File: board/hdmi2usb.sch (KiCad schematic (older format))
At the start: 0 parts

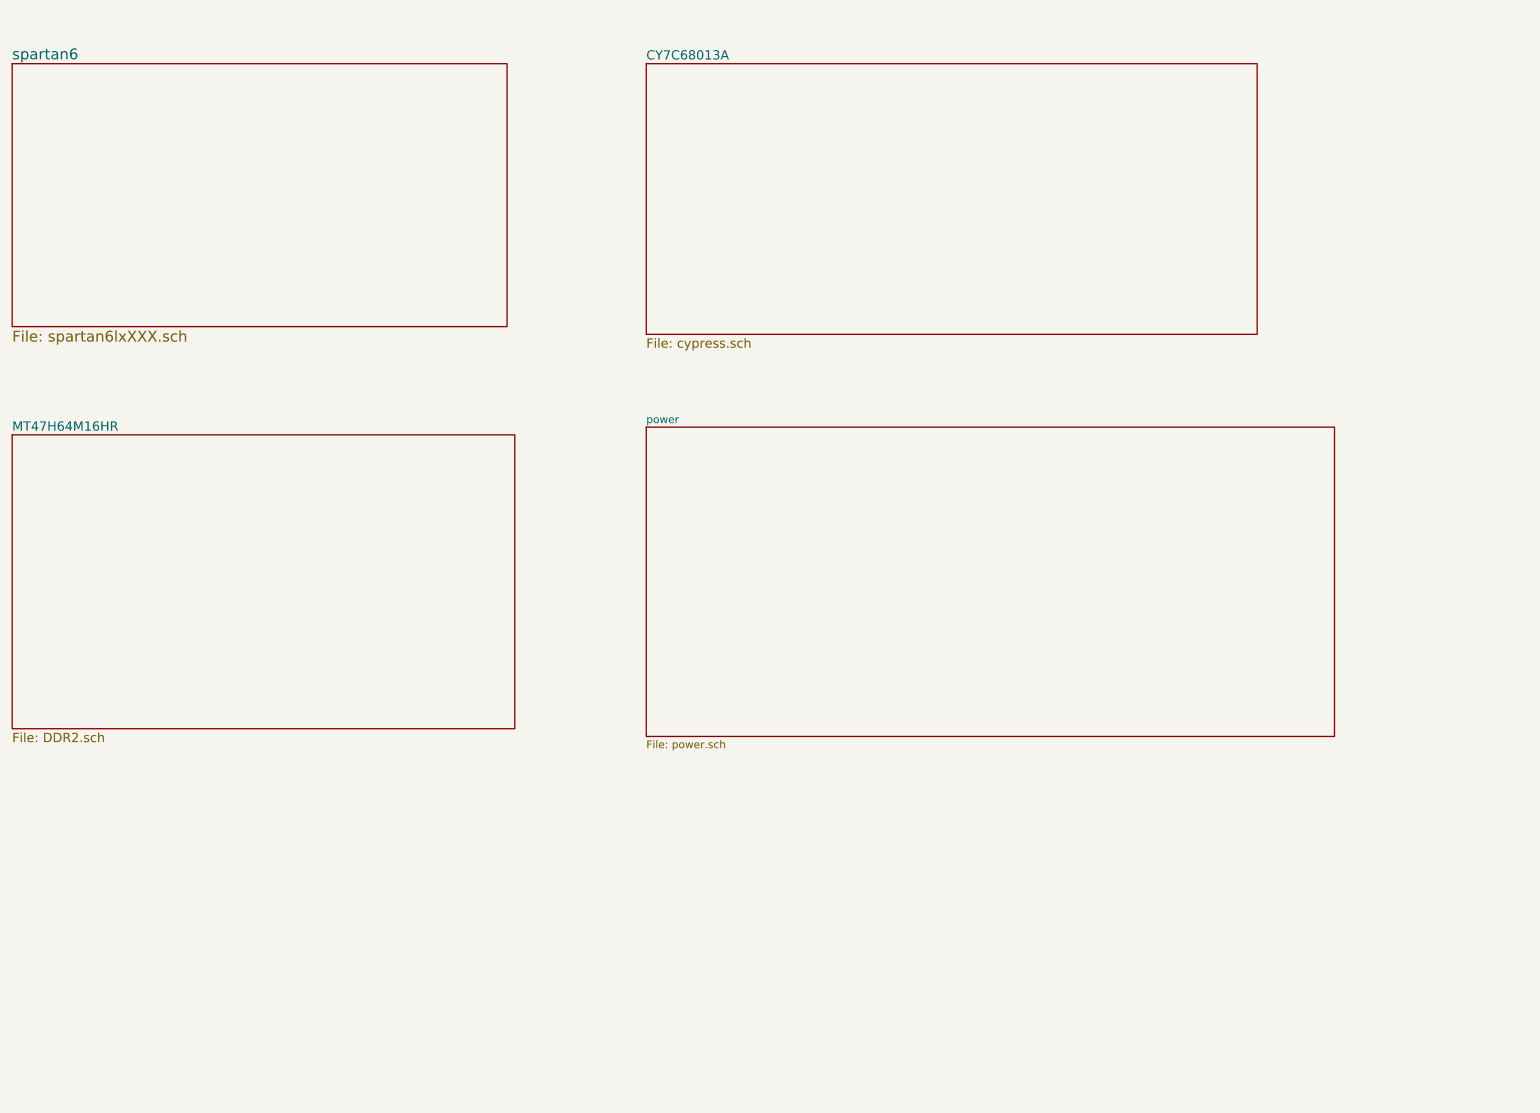
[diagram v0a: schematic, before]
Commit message: Issue #336
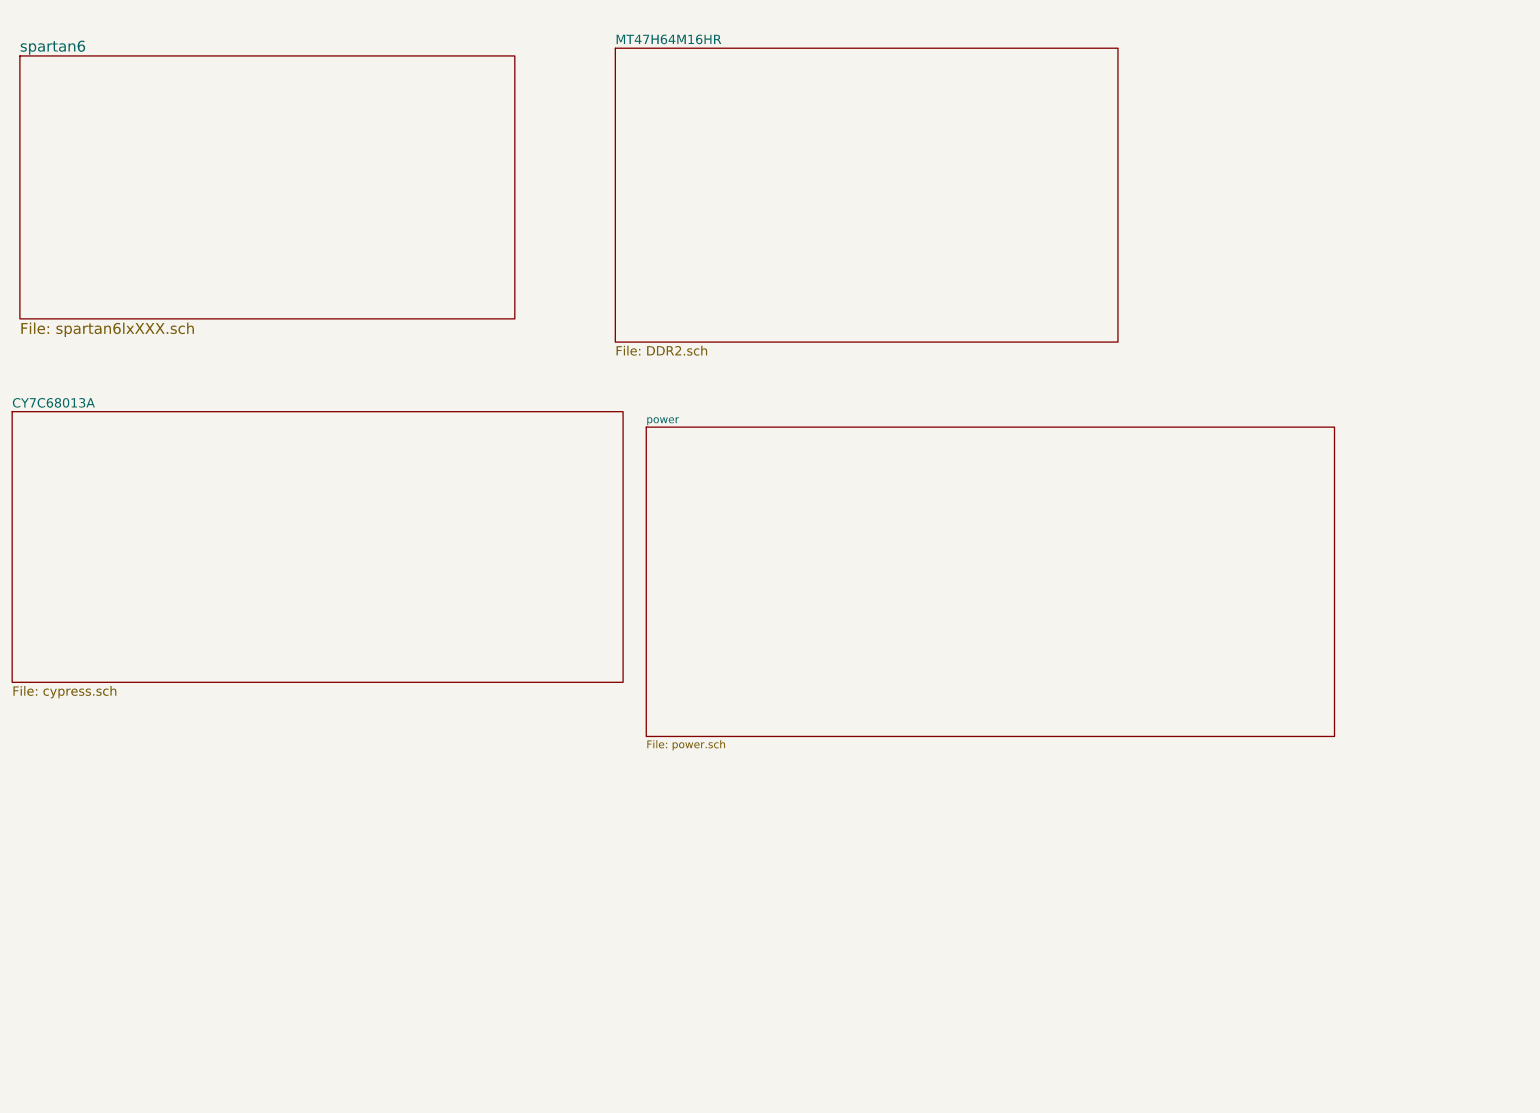
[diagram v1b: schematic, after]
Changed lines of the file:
@@
 Sheet 1 5
 Title ""
-Date "15 jun 2013"
+Date "19 jun 2013"
 Rev ""
 Comp ""
@@
 $EndDescr
 $Sheet
-S 1000 3300 3250 1900
+S 4900 800  3250 1900
 U 51B846F4
 F0 "MT47H64M16HR" 60
@@
 $EndSheet
 $Sheet
-S 5100 900  3950 1750
+S 1000 3150 3950 1750
 U 51B5BBC1
 F0 "CY7C68013A" 60
@@
 $EndSheet
 $Sheet
-S 1000 900  3200 1700
+S 1050 850  3200 1700
 U 51AED6DE
 F0 "spartan6" 70

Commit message: Issue #336
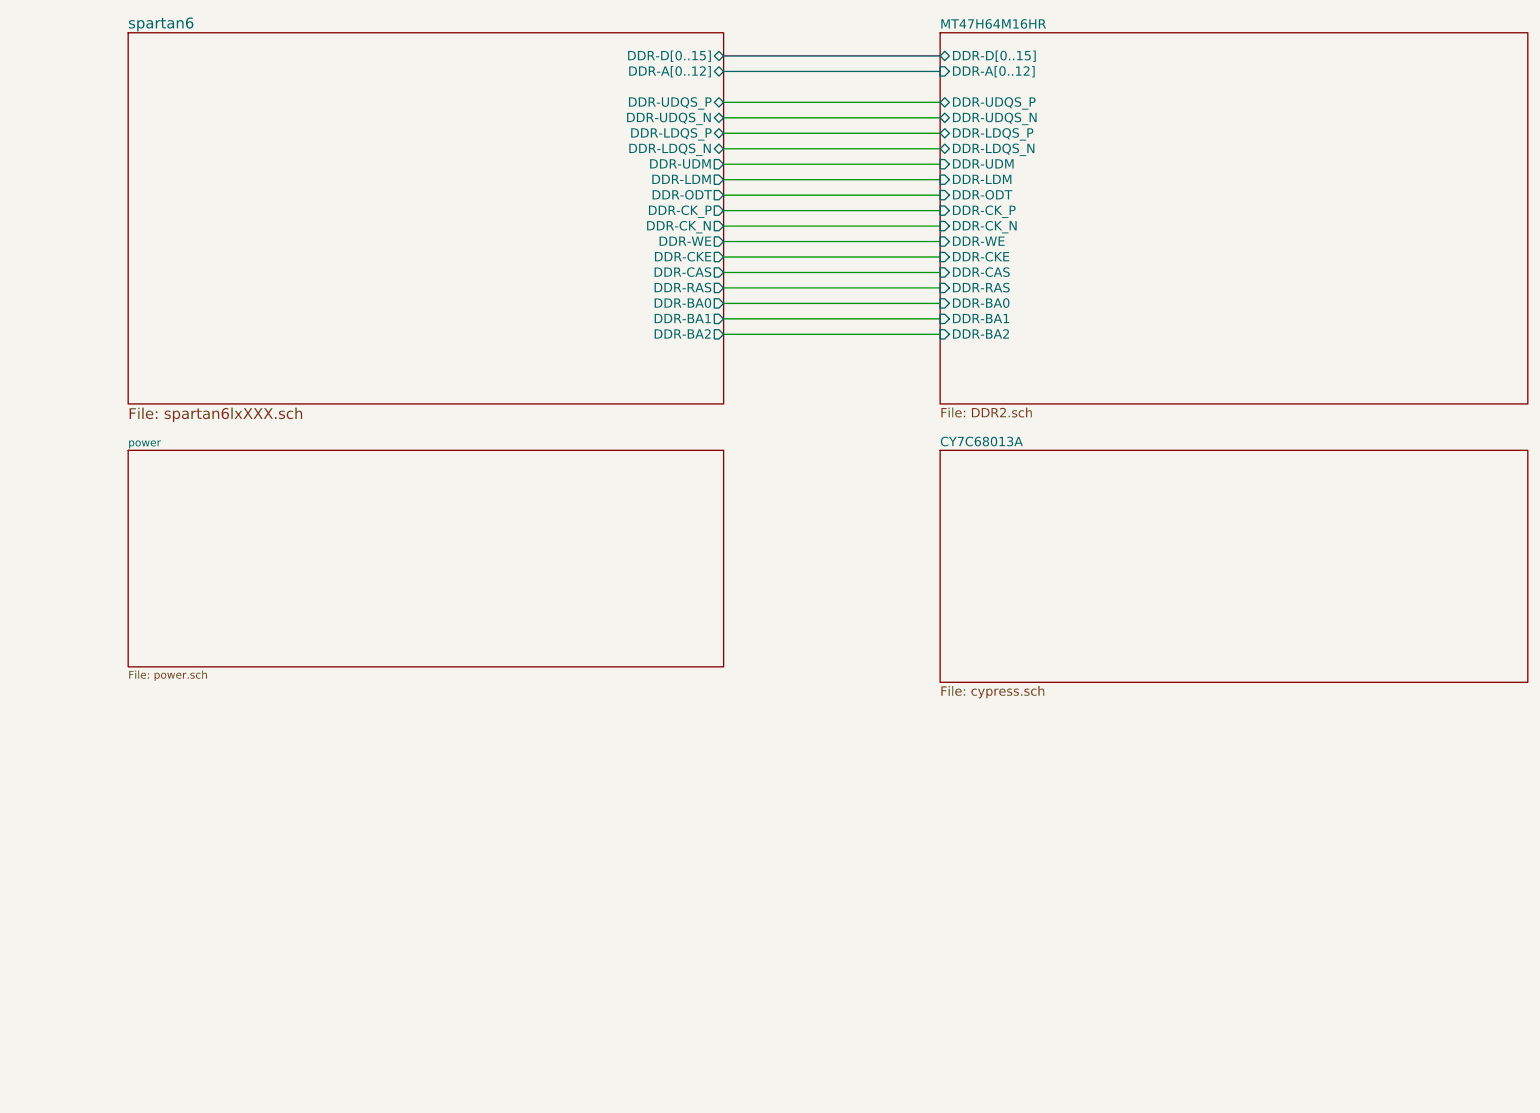
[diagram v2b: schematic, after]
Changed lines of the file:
@@
 Sheet 1 5
 Title ""
-Date "19 jun 2013"
+Date "24 jun 2013"
 Rev ""
 Comp ""
@@
 $EndDescr
 $Sheet
-S 4900 800  3250 1900
-U 51B846F4
-F0 "MT47H64M16HR" 60
-F1 "DDR2.sch" 60
-$EndSheet
-$Sheet
-S 1000 3150 3950 1750
+S 7000 3400 3800 1500
 U 51B5BBC1
 F0 "CY7C68013A" 60
@@
 $EndSheet
 $Sheet
-S 1050 850  3200 1700
-U 51AED6DE
-F0 "spartan6" 70
-F1 "spartan6lxXXX.sch" 70
-$EndSheet
-$Sheet
-S 5100 3250 4450 2000
+S 1750 3400 3850 1400
 U 51BACC6F
 F0 "power" 50
 F1 "power.sch" 50
 $EndSheet
+Wire Bus Line
+	7000 850  5600 850
+Wire Bus Line
+	7000 950  5600 950
+$Sheet
+S 7000 700  3800 2400
+U 51B846F4
+F0 "MT47H64M16HR" 60
+F1 "DDR2.sch" 60
+F2 "DDR-D[0..15]" B L 7000 850 60
+F3 "DDR-A[0..12]" I L 7000 950 60
+F4 "DDR-UDQS_P" B L 7000 1150 60
+F5 "DDR-UDQS_N" B L 7000 1250 60
+F6 "DDR-LDQS_P" B L 7000 1350 60
+F7 "DDR-LDQS_N" B L 7000 1450 60
+F8 "DDR-UDM" I L 7000 1550 60
+F9 "DDR-LDM" I L 7000 1650 60
+F10 "DDR-ODT" I L 7000 1750 60
+F11 "DDR-CK_P" I L 7000 1850 60
+F12 "DDR-CK_N" I L 7000 1950 60
+F13 "DDR-CKE" I L 7000 2150 60
+F14 "DDR-WE" I L 7000 2050 60
+F15 "DDR-CAS" I L 7000 2250 60
+F16 "DDR-RAS" I L 7000 2350 60
+F17 "DDR-BA0" I L 7000 2450 60
+F18 "DDR-BA1" I L 7000 2550 60
+F19 "DDR-BA2" I L 7000 2650 60
+$EndSheet
+$Sheet
+S 1750 700  3850 2400
+U 51AED6DE
+F0 "spartan6" 70
+F1 "spartan6lxXXX.sch" 70
+F2 "DDR-D[0..15]" B R 5600 850 60
+F3 "DDR-A[0..12]" B R 5600 950 60
+F4 "DDR-LDQS_P" B R 5600 1350 60
+F5 "DDR-LDQS_N" B R 5600 1450 60
+F6 "DDR-UDM" O R 5600 1550 60
+F7 "DDR-LDM" O R 5600 1650 60
+F8 "DDR-UDQS_P" B R 5600 1150 60
+F9 "DDR-UDQS_N" B R 5600 1250 60
+F10 "DDR-RAS" O R 5600 2350 60
+F11 "DDR-CAS" O R 5600 2250 60
+F12 "DDR-ODT" O R 5600 1750 60
+F13 "DDR-CK_P" O R 5600 1850 60
+F14 "DDR-CK_N" O R 5600 1950 60
+F15 "DDR-BA0" O R 5600 2450 60
+F16 "DDR-BA1" O R 5600 2550 60
+F17 "DDR-WE" O R 5600 2050 60
+F18 "DDR-BA2" O R 5600 2650 60
+F19 "DDR-CKE" O R 5600 2150 60
+$EndSheet
+Wire Wire Line
+	5600 1150 7000 1150
+Wire Wire Line
+	7000 1250 5600 1250
+Wire Wire Line
+	5600 1350 7000 1350
+Wire Wire Line
+	7000 1450 5600 1450
+Wire Wire Line
+	5600 1550 7000 1550
+Wire Wire Line
+	7000 1650 5600 1650
+Wire Wire Line
+	5600 1750 7000 1750
+Wire Wire Line
+	7000 1850 5600 1850
+Wire Wire Line
+	5600 1950 7000 1950
+Wire Wire Line
+	5600 2050 7000 2050
+Wire Wire Line
+	5600 2150 7000 2150
+Wire Wire Line
+	7000 2250 5600 2250
+Wire Wire Line
+	5600 2350 7000 2350
+Wire Wire Line
+	5600 2450 7000 2450
+Wire Wire Line
+	7000 2550 5600 2550
+Wire Wire Line
+	5600 2650 7000 2650
 $EndSCHEMATC
